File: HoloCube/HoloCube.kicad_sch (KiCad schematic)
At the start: 26 parts, among them J1 ESPProgUART_RX, J2 Conn_01x08_MountingPin, J3 USB_C_Receptacle_USB2.0, U1 ESP32-PICO-D4, U2 LIS2DE12, U3 BH1750FVI-TR, U4 XC6209

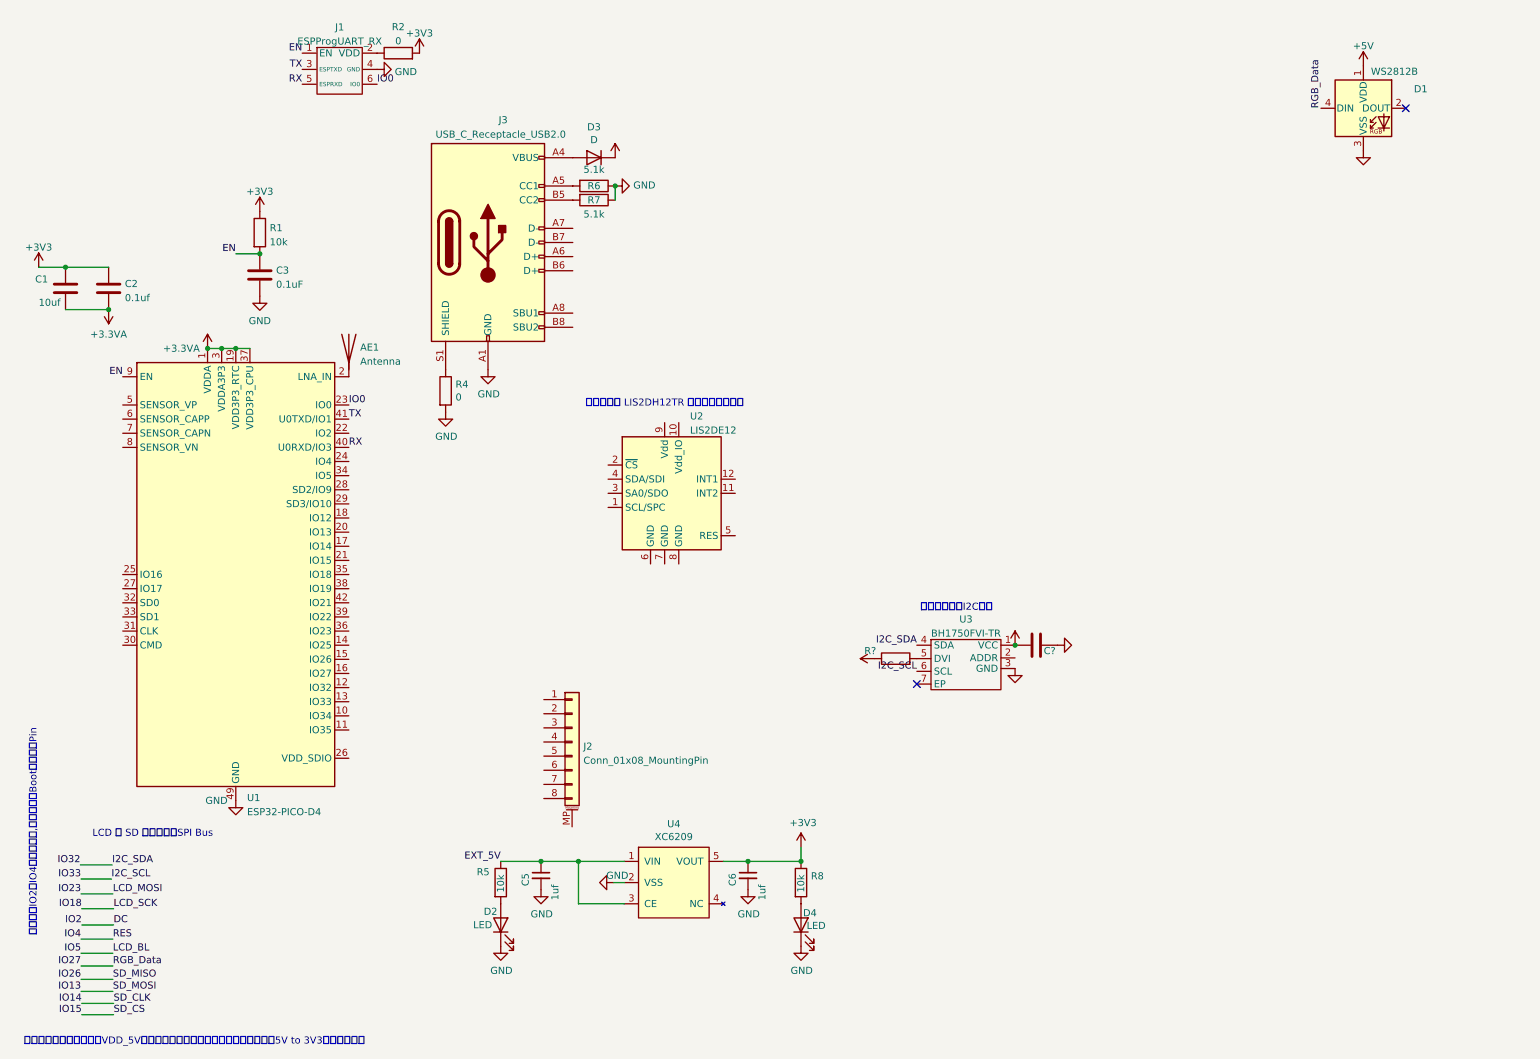
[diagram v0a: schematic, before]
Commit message: Place Parts
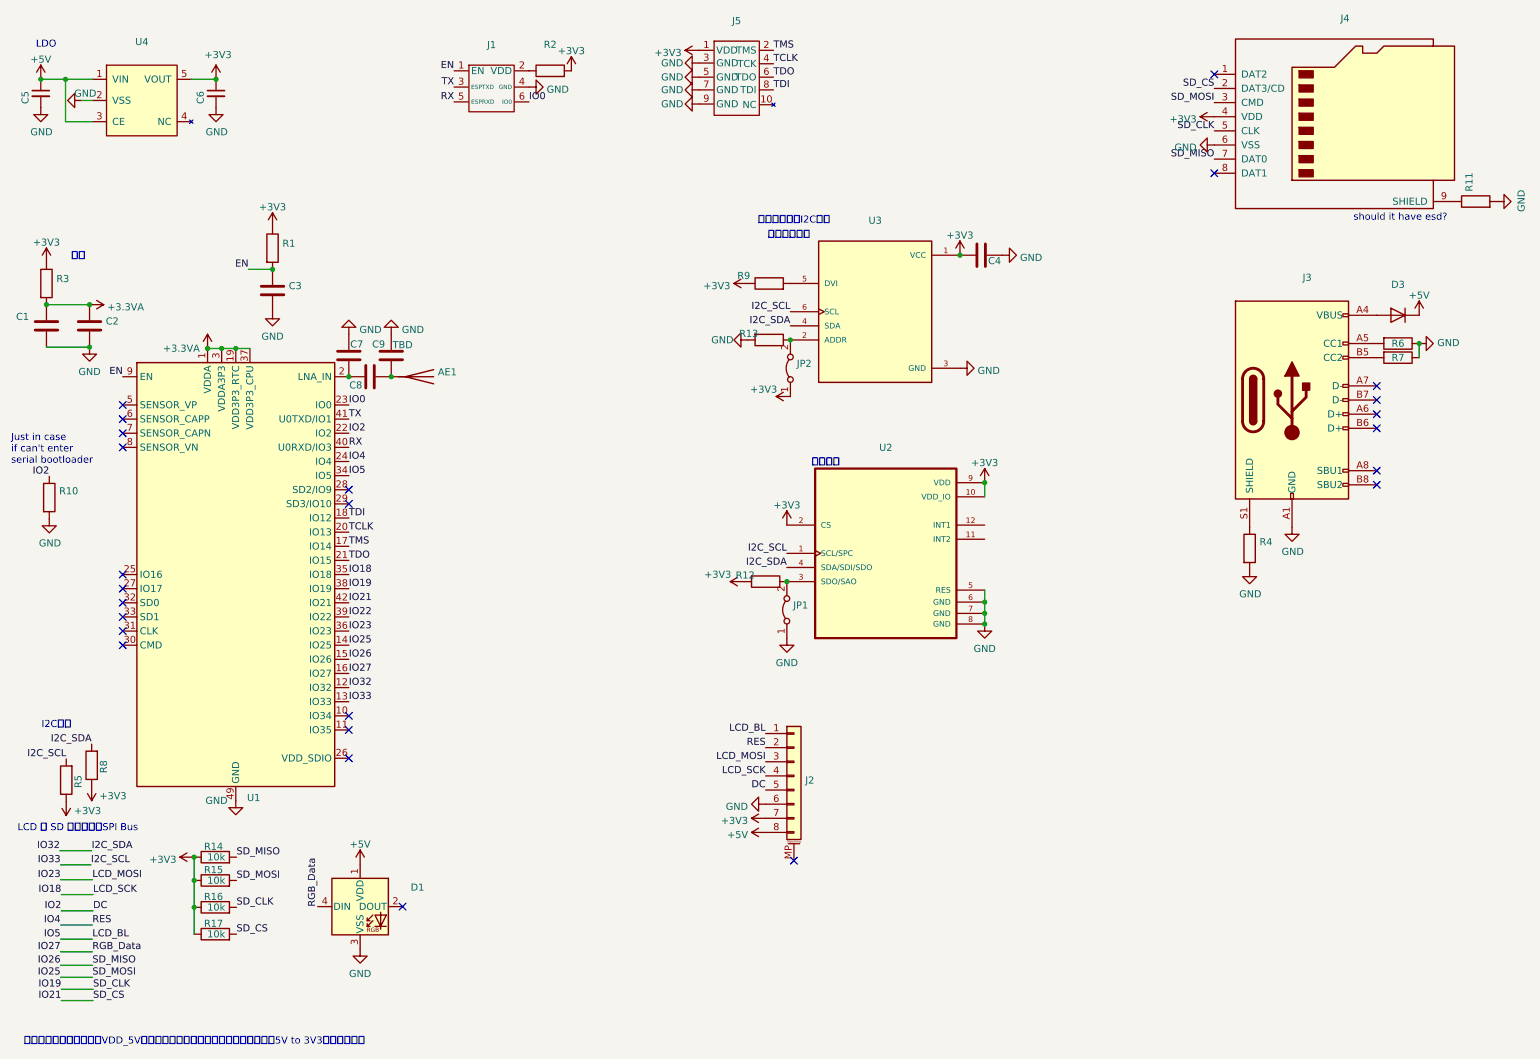
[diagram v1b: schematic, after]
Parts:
- removed C?: (no value), symbol Device:C
- removed D2, D4: LED, LED_SMD:LED_0603_1608Metric, symbol Device:LED
- removed R?: (no value), symbol Device:R
- removed U2: LIS2DE12, Package_LGA:LGA-12_2x2mm_P0.5mm, symbol Sensor_Motion:LIS2DE12
- removed U3: BH1750FVI-TR, symbol KisonNew:BH1750FVI-TR
- added C4: (no value), symbol Device:C
- added C7, C8: (no value), Capacitor_SMD:C_0603_1608Metric, symbol Device:C
- added C9: TBD, Capacitor_SMD:C_0603_1608Metric, symbol Device:C
- added J4: (no value), symbol Connector:Micro_SD_Card
- added J5: (no value), symbol KisonNew:ESPProgJTAG_RX
- added JP1, JP2: (no value), symbol Jumper:Jumper_2_Bridged
- added R10, R11, R12, R13, R3, R9: (no value), symbol Device:R
- added R14, R15, R16, R17: 10k, Resistor_SMD:R_0603_1608Metric, symbol Device:R
- added U2: (no value), symbol LIS2DH12TR:LIS2DH12TR
- added U3: (no value), symbol BH1750FVI-TR:BH1750FVI-TR
- AE1: value Antenna -> (none); footprint RF_Antenna:Texas_SWRA117D_2.4GHz_Right -> (none)
- C1: value 10uf -> (none)
- C2: value 0.1uf -> (none)
- C3: value 0.1uF -> (none); footprint Capacitor_SMD:C_0603_1608Metric -> (none)
- C5, C6: value 1uf -> (none); footprint Capacitor_SMD:C_0603_1608Metric -> (none)
- D1: value WS2812B -> (none); footprint LED_SMD:LED_WS2812B_PLCC4_5.0x5.0mm_P3.2mm -> (none)
- D3: value D -> (none); footprint KisonNew:C8678 -> (none)
- J1: value ESPProgUART_RX -> (none); footprint KisonNew:IDC_1.27mm_6P -> (none)
- J2: value Conn_01x08_MountingPin -> (none)
- J3: value USB_C_Receptacle_USB2.0 -> (none); footprint Connector_USB:USB_C_Receptacle_HRO_TYPE-C-31-M-12 -> (none)
- R1: value 10k -> (none); footprint Resistor_SMD:R_0603_1608Metric -> (none)
- R2: value 0 -> (none)
- R4: value 0 -> (none); footprint Resistor_SMD:R_0603_1608Metric -> (none)
- R5, R8: value 10k -> (none); footprint Resistor_SMD:R_0603_1608Metric -> (none); LCSC (none) -> C429617
- R6, R7: value 5.1k -> (none); footprint Resistor_SMD:R_0603_1608Metric -> (none)
- U1: value ESP32-PICO-D4 -> (none); footprint Package_DFN_QFN:QFN-48-1EP_7x7mm_P0.5mm_EP5.3x5.3mm -> (none)
- U4: value XC6209 -> (none); footprint Package_TO_SOT_SMD:SOT-23-5 -> (none)
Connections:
- net +3.3VA: now also C1.1, C2.1, R3.2; no longer C1.2, C2.2
- net +3V3: now also J2.7 (Pin_7), R5.1, C4.1, J4.4 (VDD), J5.1 (VDD), JP2.1 (A), R12.2, R14.1, R15.1, R16.1, R17.1, R3.1, R9.1, U2.10 (VDD_IO), U2.2 (CS), U2.9 (VDD), U3.1 (VCC); no longer C1.1, C2.1
- net +5V: now also C5.1, J2.8 (Pin_8), U4.1 (VIN), U4.3 (CE)
- net DC: now also J2.5 (Pin_5), U1.22 (IO2), R10.1
- net GND: now also C1.2, C2.2, J2.6 (Pin_6), C4.2, C7.1, C9.1, J4.6 (VSS), J5.3 (GND), J5.5 (GND), J5.7 (GND), J5.9 (GND), JP1.1 (A), R10.2, R11.2, R13.2, U2.5 (RES), U2.6 (GND), U2.7 (GND), U2.8 (GND), U3.3 (GND)
- net I2C_SCL: now also R5.2, U1.13 (IO33), U2.1 (SCL/SPC), U3.6 (SCL)
- net I2C_SDA: now also R8.2, U1.12 (IO32), U2.4 (SDA/SDI/SDO), U3.4 (SDA)
- net IO18: now also J2.4 (Pin_4), U1.35 (IO18)
- net IO23: now also J2.3 (Pin_3), U1.36 (IO23)
- net IO26: now also U1.15 (IO26), J4.7 (DAT0), R14.2
- net IO27: now also U1.16 (IO27)
- net IO4: now also J2.2 (Pin_2), U1.24 (IO4)
- net IO5: now also J2.1 (Pin_1), U1.34 (IO5)
- net at AE1.1 (A): now also C8.2, C9.2; no longer U1.2 (LNA_IN)
- net IO25: now reaches U1.14 (IO25)
- net IO25: now also J4.3 (CMD), R15.2
- net TMS: now reaches U1.17 (IO14)
- net TMS: now also J5.2 (TMS)
- net TDI: now reaches U1.18 (IO12)
- net TDI: now also J5.8 (TDI)
- net TCLK: now reaches U1.20 (IO13)
- net TCLK: now also J5.4 (TCK)
- net TDO: now reaches U1.21 (IO15)
- net TDO: now also J5.6 (TDO)
- net IO19: now reaches U1.38 (IO19)
- net IO19: now also J4.5 (CLK), R16.2
- net IO22: now reaches U1.39 (IO22)
- net IO21: now reaches U1.42 (IO21)
- net IO21: now also J4.2 (DAT3/CD), R17.2
- removed net EXT_5V: C5.1, R5.1, U4.1 (VIN), U4.3 (CE)
- new net: J4.9 (SHIELD), R11.1
- new net: JP2.2 (B), R13.1, U3.2 (ADDR)
- new net: R9.2, U3.5 (DVI)
- new net: JP1.2 (B), R12.1, U2.3 (SDO/SAO)
- new net: C7.2, C8.1, U1.2 (LNA_IN)
- no-connect marks 2 -> 25
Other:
- note added: "I2C上拉"
- note added: "Just in case if can't enter serial bootloader"
- note added: "LDO"
- note added: "should it have esd?"
- note added: "加速度计"
- note added: "滤波"
- note added: "环境光传感器"
- note removed: "注意检查IO2与IO4的设计要求,确保不影响Boot或直接换Pin"
- note removed: "注意检查与 LIS2DH12TR 的区别，别忘了（"
- moved on the sheet: AE1, C1, C2, C3, C5, C6, D1, D3, J1, J2, J3, R1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
